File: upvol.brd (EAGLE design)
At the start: 30.8 x 20.2 mm, 11 parts, among them IC1 LM393D, J1 61300311121, J2 61300211121

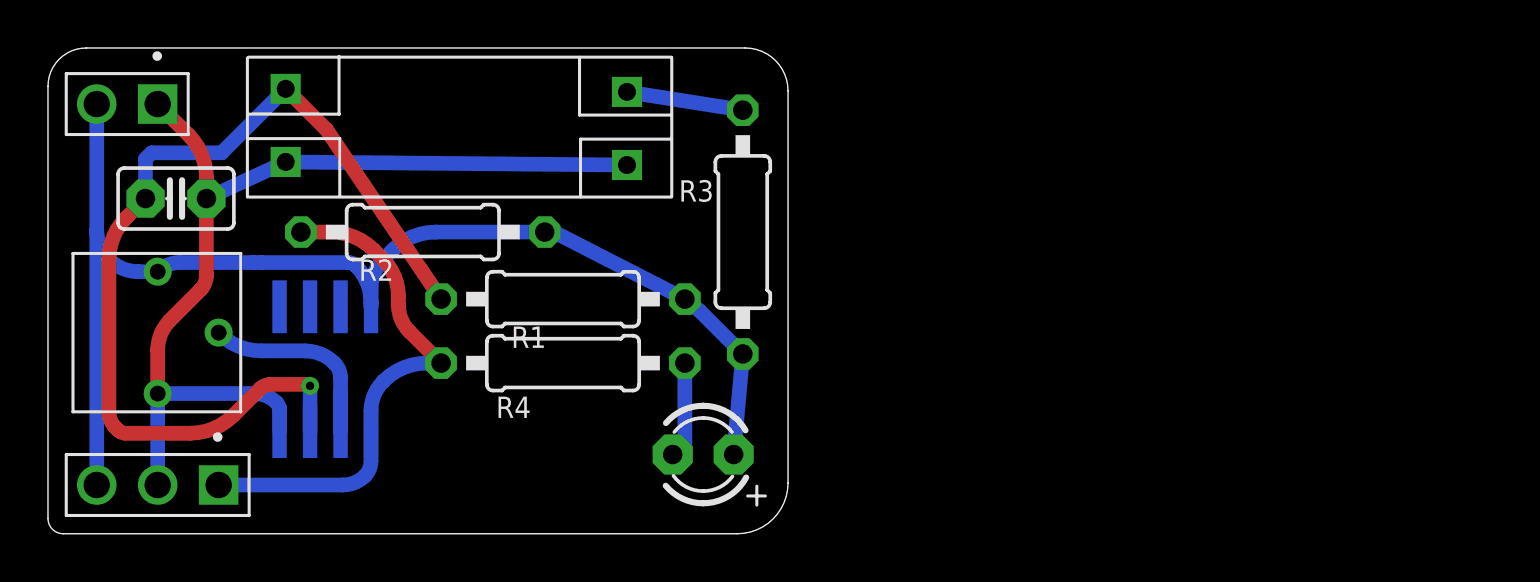
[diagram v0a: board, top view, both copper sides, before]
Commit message: add
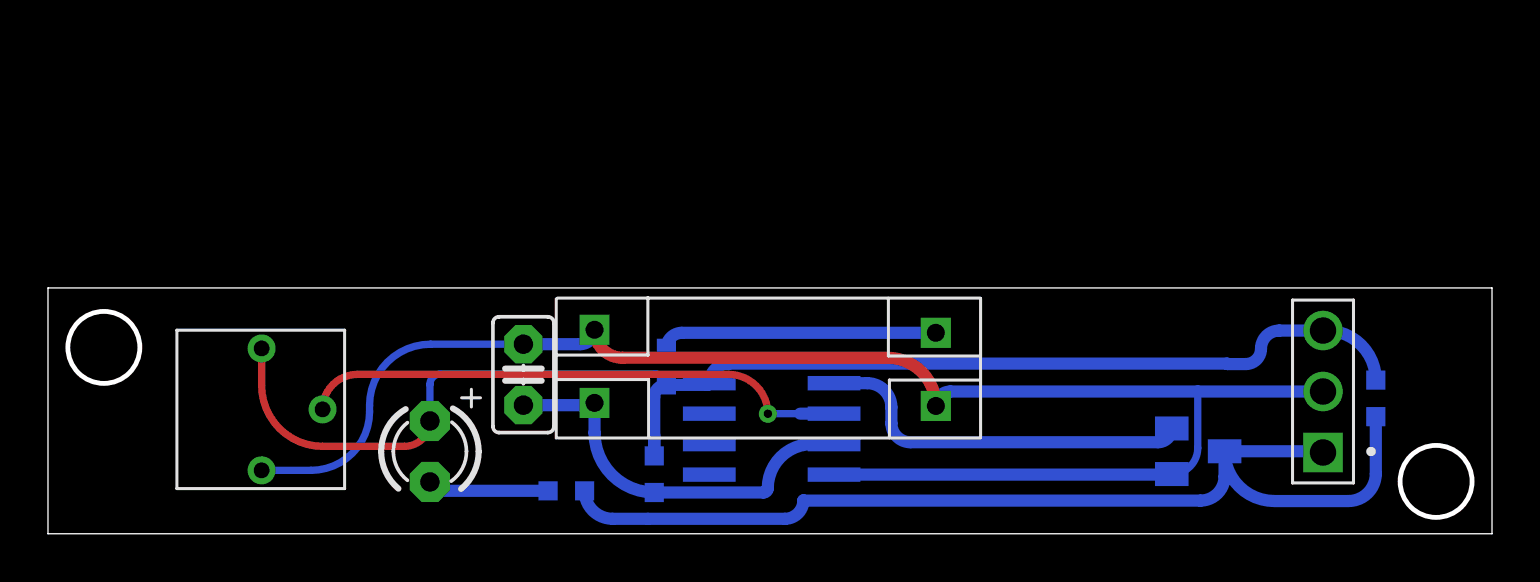
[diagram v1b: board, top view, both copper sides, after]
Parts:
- removed J2: 61300211121, Headers:61300211121
- added T1: s9014, transistor:SOT23-EBC
- R1, R2, R4: device OPL_Resistor:PR-D2.3XL6.5MM -> 52101-101-REV-A_v16:RC-MASTER-SMD_R0603MP
- R3: value 100 -> 4.7k; device OPL_Resistor:PR-D2.3XL6.5MM -> 52101-101-REV-A_v16:RC-MASTER-SMD_R0603MP
- moved J1 48.7 mm to (53.1, 5.93), turned to 90 degrees
- moved R2 40.4 mm to (55.3, 5.64), flipped to the bottom, turned to 90 degrees
- moved IC1 18.8 mm to (30.2, 4.37), turned to 270 degrees
- moved U$1 16.3 mm to (30.3, 6.85)
- moved C1 16.2 mm to (19.8, 6.63), turned to 270 degrees
- moved LED1 11.4 mm to (15.9, 3.43), turned to 270 degrees
- moved R1 8.29 mm to (25.3, 2.48), flipped to the bottom, turned to 90 degrees
- moved R3 6.56 mm to (25.8, 6.97), flipped to the bottom
- moved R5 5.38 mm to (8.90, 5.18)
- moved R4 5.33 mm to (21.6, 1.79), flipped to the bottom
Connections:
- new net N$5: IC1.1, T1.B
- net N$1: now also C1.2, U$1.C; no longer C1.1, U$1.E
- net OUT: now also T1.C; no longer IC1.1
- net V+: no longer J2.2
- net V-: now also C1.1, T1.E, U$1.E; no longer C1.2, J2.1, U$1.C
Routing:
- net V-: track 41.4 -> 66.4 mm
- net N$1: track 40.5 -> 16.1 mm, vias 1 -> 0
- net OUT: track 21.7 -> 43.1 mm
- net N$5: track 0.00 -> 15.7 mm
- net N$4: track 9.60 -> 22.6 mm, vias 0 -> 1
- net N$2: track 4.89 -> 11.5 mm
- net V+: track 52.7 -> 57.7 mm
- net N$3: track 4.02 -> 5.08 mm
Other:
- board size 30.8 x 20.2 mm -> 60.2 x 10.2 mm
